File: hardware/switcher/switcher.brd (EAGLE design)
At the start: 55 x 82 mm, 9 parts, among them IC1 L293E

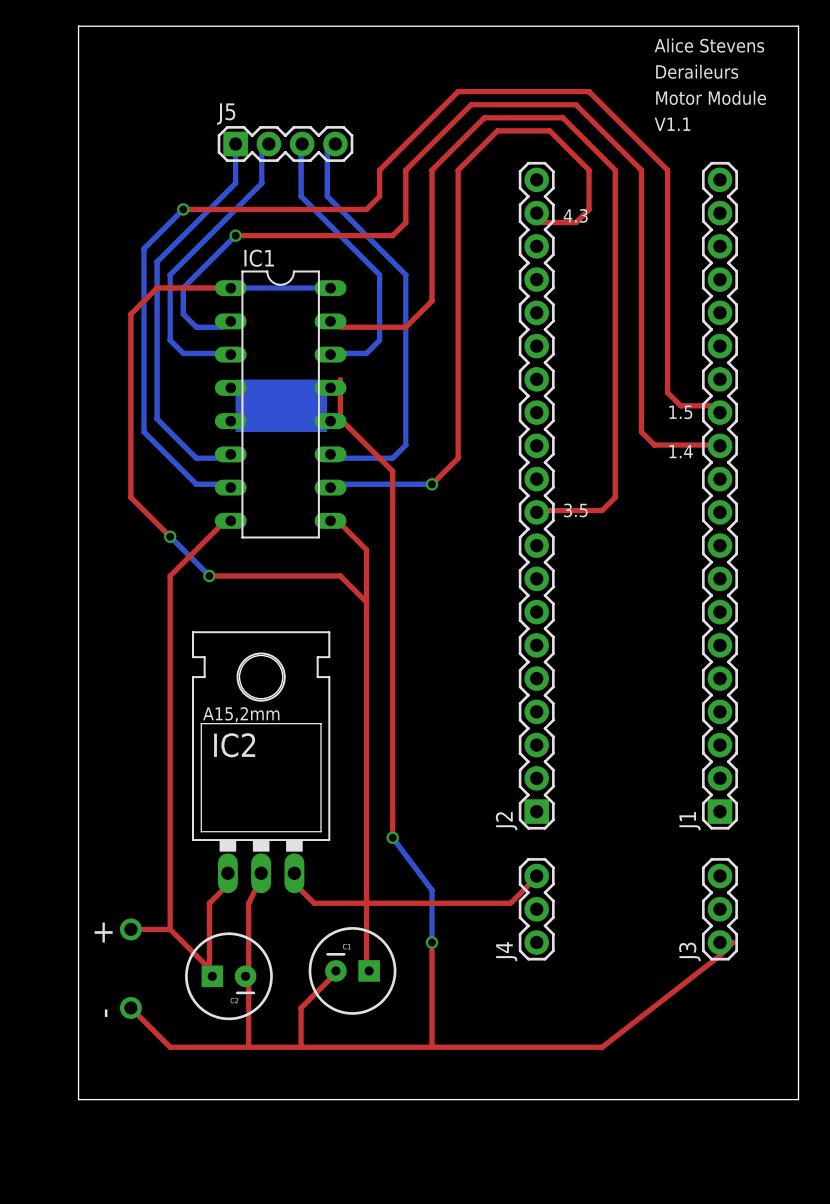
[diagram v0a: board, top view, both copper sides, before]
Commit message: finish boards
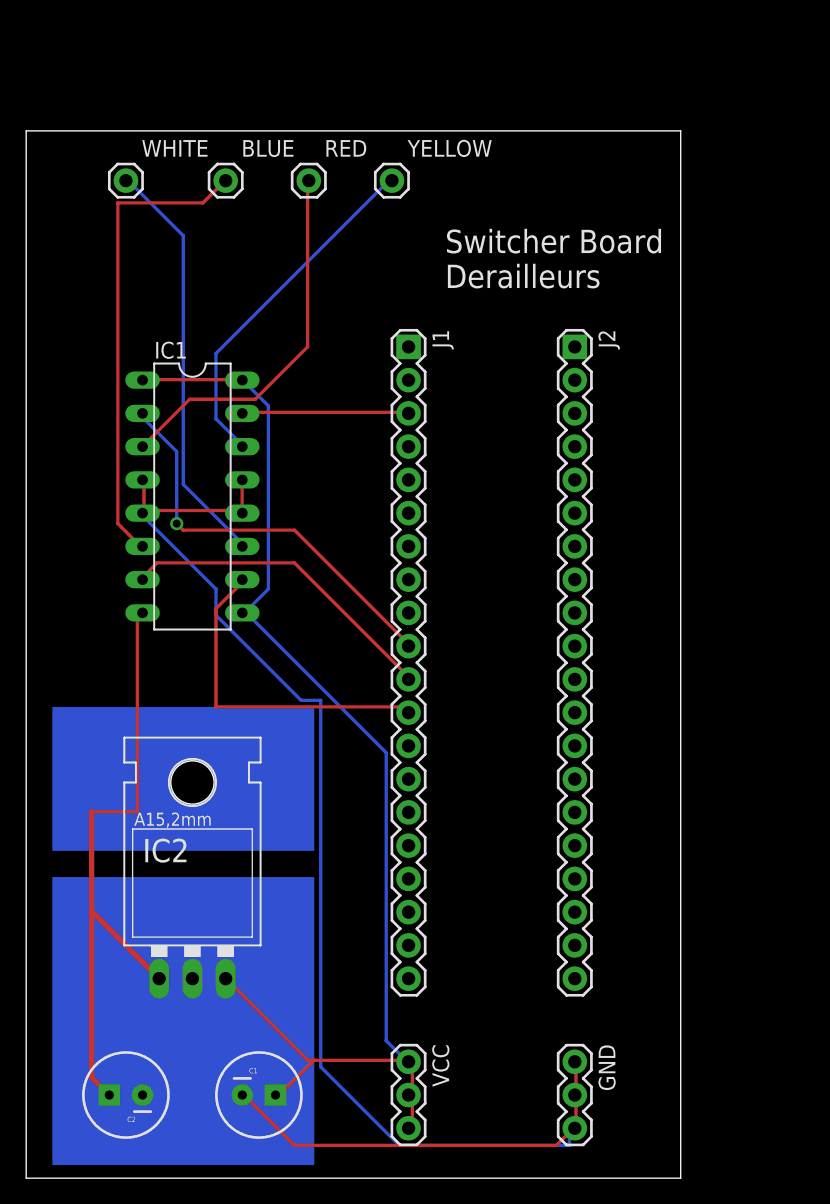
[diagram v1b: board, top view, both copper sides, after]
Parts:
- removed J3, J4: (no value), SparkFun-Connectors:1X03
- removed J5: (no value), SparkFun-Connectors:1X04
- added BLUE, RED, WHITE, YELLOW: (no value), SparkFun-Connectors:1X01
- added GND, VCC: (no value), SparkFun-Connectors:1X03
- moved J1 42.7 mm to (29.2, 63.5), turned to 270 degrees
- moved J2 35.6 mm to (41.9, 63.5), turned to 270 degrees
- moved C2 12.0 mm to (7.62, 6.35)
- moved C1 11.9 mm to (17.8, 6.35)
- moved IC1 9.74 mm to (12.7, 52.1)
- moved IC2 9.61 mm to (12.7, 19.1)
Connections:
- removed net P2.4: IC1.15
- new net P2.5: IC1.15, J1.3
- net GND: now also GND.1, GND.2, GND.3
- net MOTOR-BLUE: now also BLUE.1
- net MOTOR-RED: now also RED.1
- net MOTOR-WHITE: now also WHITE.1
- net MOTOR-YELLOW: now also YELLOW.1
- net P3.4: now also J1.10
- net P3.5: now also J1.11
- net P3.6: now also J1.12
- net VCC: now also VCC.1, VCC.2, VCC.3
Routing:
- net GND: track 0.00 -> 132.9 mm
- net N$6: track 116.0 -> 0.00 mm, vias 3 -> 0
- net N$16: track 98.6 -> 0.00 mm, vias 2 -> 0
- net VCC: track 0.00 -> 93.1 mm
- net N$14: track 91.7 -> 0.00 mm, vias 1 -> 0
- net N$11: track 77.0 -> 0.00 mm, vias 1 -> 0
- net N$7: track 66.6 -> 0.00 mm
- net N$13: track 51.7 -> 0.00 mm, vias 1 -> 0
- net 9V: track 0.00 -> 48.4 mm
- net N$3: track 47.7 -> 0.00 mm, vias 1 -> 0
- net MOTOR-BLUE: track 0.00 -> 36.0 mm
- net MOTOR-WHITE: track 0.00 -> 31.7 mm
- net P3.4: track 0.00 -> 31.1 mm, vias 0 -> 1
- net N$10: track 30.9 -> 0.00 mm
- net N$15: track 29.7 -> 0.00 mm
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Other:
- board size 55 x 82 mm -> 50 x 80 mm
- board text added: "Switcher Board Derailleurs"
- board text removed: "+"
- board text removed: "-"
- board text removed: "1.4"
- board text removed: "1.5"
- board text removed: "3.5"
- board text removed: "4.3"
- board text removed: "Alice Stevens"
- board text removed: "BLUE"
- board text removed: "Deraileurs"
- board text removed: "Motor Module"
- board text removed: "RED"
- board text removed: "V1.1"
- board text removed: "WHITE"
- board text removed: "YELLOW"
